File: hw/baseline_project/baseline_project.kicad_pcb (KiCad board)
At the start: 2 copper layers, 115 x 94 mm, 17 parts, among them J101 EXT_3V3, Q101 IRLD024PBF, SW101 UP, SW102 DOWN, SW103 LEFT, SW104 RIGHT, SW105 MODE, U101 EK-TM4C123GXL, U102 ESP8266-01/ESP-01, U103 Adafruit ST7735R

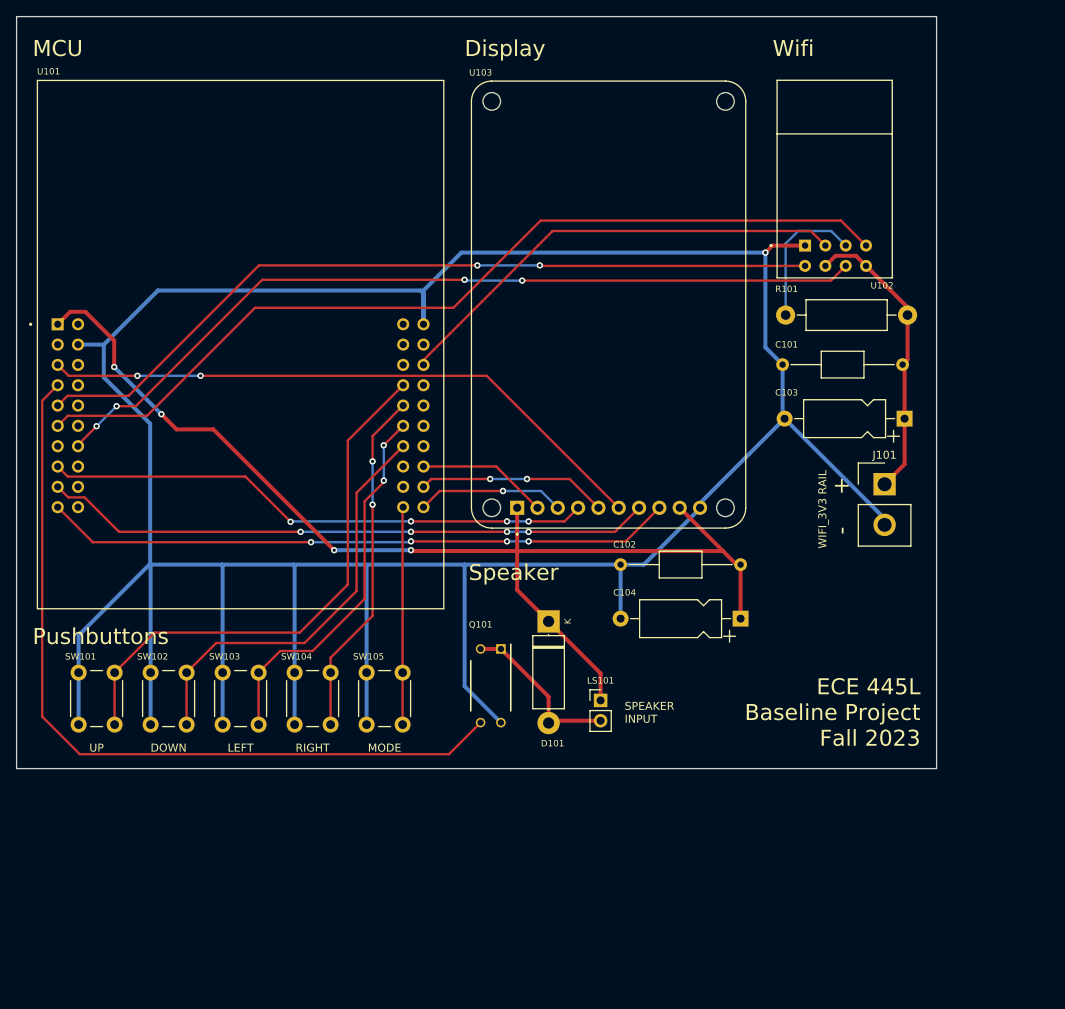
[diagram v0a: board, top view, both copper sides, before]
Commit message: SchematicDone
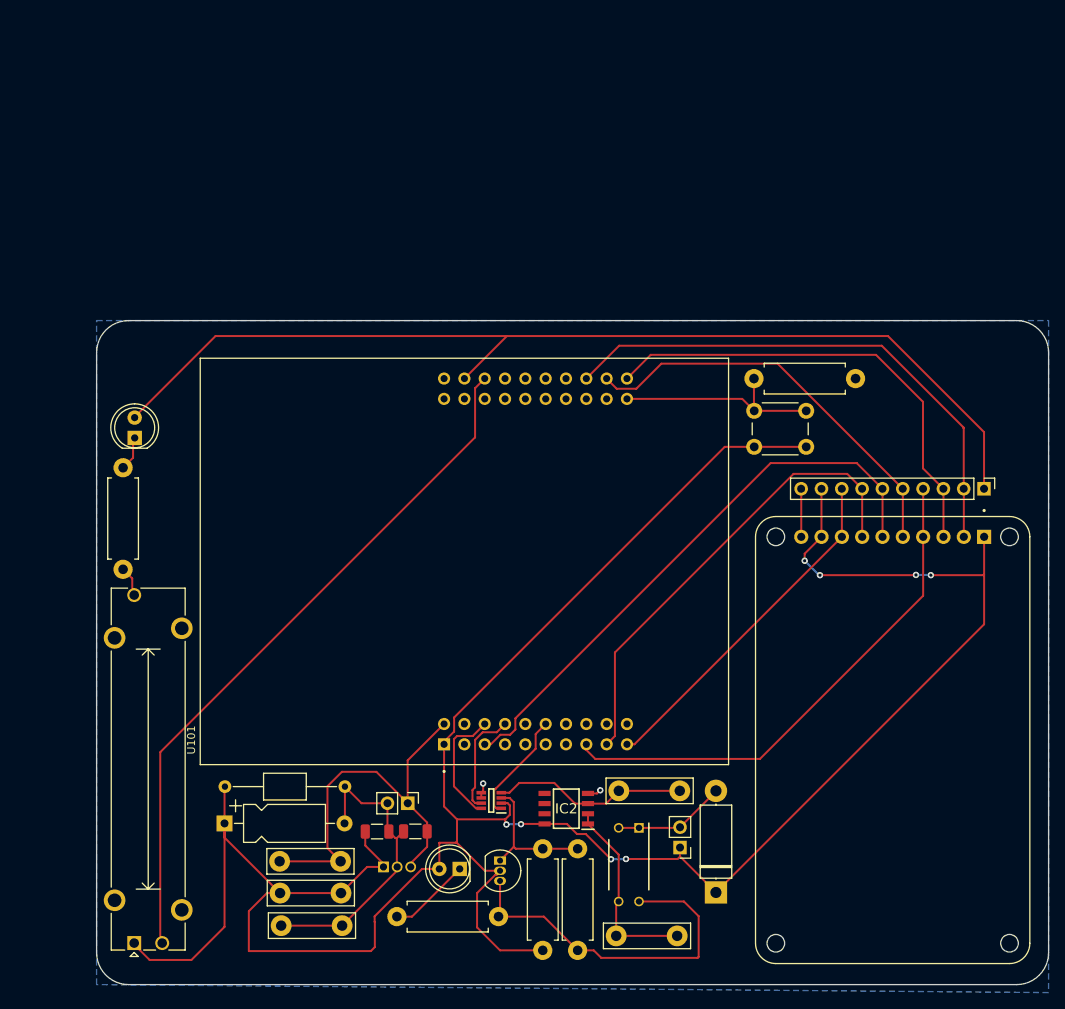
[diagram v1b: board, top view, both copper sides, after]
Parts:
- removed C101: 100nF, Capacitor_THT:C_Axial_L5.1mm_D3.1mm_P15.00mm_Horizontal
- removed C103: 4.7uF, Capacitor_THT:CP_Axial_L10.0mm_D4.5mm_P15.00mm_Horizontal
- removed J101: EXT_3V3, Connector_Samtec_HPM_THT:Samtec_HPM-02-01-x-S_Straight_1x02_Pitch5.08mm
- removed R101: 10k, Resistor_THT:R_Axial_DIN0411_L9.9mm_D3.6mm_P15.24mm_Horizontal
- removed SW101: UP, Button_Switch_THT:SW_PUSH_6mm
- removed SW102: DOWN, Button_Switch_THT:SW_PUSH_6mm
- removed SW103: LEFT, Button_Switch_THT:SW_PUSH_6mm
- removed SW104: RIGHT, Button_Switch_THT:SW_PUSH_6mm
- removed SW105: MODE, Button_Switch_THT:SW_PUSH_6mm
- removed U102: ESP8266-01/ESP-01, footprints:ai_thinker_ESP8266_01
- added C1: 1u, Capacitor_SMD:C_1206_3216Metric, F.Cu at (81.8, 132.8)
- added C2: 1u, Capacitor_SMD:C_1206_3216Metric, F.Cu at (77.1, 132.9)
- added D1: LED, LED_THT:LED_D5.0mm, F.Cu at (46.8, 83.7)
- added D2: LED, LED_THT:LED_D5.0mm, F.Cu at (87.4, 137.5)
- added IC1: AD5061BRJZ-1500RL7, footprints:SOT65P280X145-8N, F.Cu at (91.3, 129.0)
- added IC2: AD823ARZ, footprints:SOIC127P600X175-8N, F.Cu at (100.7, 130.0)
- added IC3: LP2950-33LPE3, footprints:TO127P419X482X788-3P, F.Cu at (78.3, 137.3)
- added J1: Logic, Connector_PinHeader_2.54mm:PinHeader_1x10_P2.54mm_Vertical, F.Cu at (152.9, 90.0)
- added J2: battery, Connector_PinHeader_2.54mm:PinHeader_1x02_P2.54mm_Vertical, F.Cu at (80.9, 129.3)
- added R1: R, Resistor_THT:R_Axial_DIN0411_L9.9mm_D3.6mm_P12.70mm_Horizontal, F.Cu at (45.3, 87.4)
- added R2: R, Resistor_THT:R_Axial_DIN0411_L9.9mm_D3.6mm_P12.70mm_Horizontal, F.Cu at (79.5, 143.5)
- added R3: R, Resistor_THT:R_Axial_DIN0411_L9.9mm_D3.6mm_P12.70mm_Horizontal, F.Cu at (97.8, 147.7)
- added R4: R, Resistor_THT:R_Axial_DIN0411_L9.9mm_D3.6mm_P12.70mm_Horizontal, F.Cu at (102.1, 135.0)
- added R5: R, Resistor_THT:R_Axial_DIN0411_L9.9mm_D3.6mm_P12.70mm_Horizontal, F.Cu at (124.2, 76.2)
- added RV1: R_Potentiometer, Potentiometer_THT:Potentiometer_Bourns_PTA3043_Single_Slide, F.Cu at (46.7, 146.8)
- added SW1: UP, Button_Switch_THT:SW_PUSH_6mm, F.Cu at (124.2, 80.3)
- added TP1: gnd, TestPoint:TestPoint_Bridge_Pitch7.62mm_Drill1.3mm, F.Cu at (65.1, 144.6)
- added TP2: 3v3, TestPoint:TestPoint_Bridge_Pitch7.62mm_Drill1.3mm, F.Cu at (64.9, 140.6)
- added TP3: vbat, TestPoint:TestPoint_Bridge_Pitch7.62mm_Drill1.3mm, F.Cu at (64.9, 136.6)
- added TP4: dacOut, TestPoint:TestPoint_Bridge_Pitch7.62mm_Drill1.3mm, F.Cu at (107.3, 127.8)
- added TP5: spkr, TestPoint:TestPoint_Bridge_Pitch7.62mm_Drill1.3mm, F.Cu at (107.0, 145.9)
- added U1: LM4041LP-ADJ, Package_TO_SOT_THT:TO-92_Inline, F.Cu at (92.4, 136.5)
- moved C102 70.2 mm to (58.0, 127.2), turned to 0 degrees
- moved C104 69.4 mm to (58.0, 131.8), turned to 0 degrees
- moved U103 65.0 mm to (141.5, 121.4), turned to -90 degrees
- moved D101 39.8 mm to (119.4, 140.5), turned to 90 degrees
- moved U101 39.0 mm to (88.0, 99.1), turned to 90 degrees
- moved Q101 28.2 mm to (108.5, 137.0)
- moved LS101 20.9 mm to (114.9, 134.9), turned to 180 degrees
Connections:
- U101 pad J1_4: /SPEAKER_GATE -> unconnected-(U101-PB1-PadJ1_4)
- U101 pad J1_5: /WIFI_TXD -> unconnected-(U101-PE4-PadJ1_5)
- U101 pad J1_6: /WIFI_RXD -> unconnected-(U101-PE5-PadJ1_6)
- U101 pad J2_2: unconnected-(U101-PB2-PadJ2_2) -> DebugOut
- U101 pad J2_3: /WIFI_IO2 -> AIN
- U101 pad J3_1: +5V -> +BATT
- U101 pad J3_3: unconnected-(U101-PD0-PadJ3_3) -> SS1_SCK
- U101 pad J3_4: unconnected-(U101-PD1-PadJ3_4) -> SS1_FS
- U101 pad J3_6: unconnected-(U101-PD3-PadJ3_6) -> SS1_MOSI
- U101 pad J3_7: /~{WIFI_RST} -> unconnected-(U101-PE1-PadJ3_7)
- U101 pad J4_4: /SW_UP -> unconnected-(U101-PC4-PadJ4_4)
- U101 pad J4_5: /SW_RIGHT -> unconnected-(U101-PC5-PadJ4_5)
- U101 pad J4_6: /SW_LEFT -> unconnected-(U101-PC6-PadJ4_6)
- U101 pad J4_7: /SW_DOWN -> unconnected-(U101-PC7-PadJ4_7)
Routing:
- net GND: track 392.9 -> 96.7 mm, vias 1 -> 2
- net +3V3: track 143.8 -> 341.3 mm, vias 4 -> 8
- net DebugOut: track 0.00 -> 130.2 mm
- net /WIFI_RXD: track 113.0 -> 0.00 mm
- net /~{WIFI_RST}: track 105.5 -> 0.00 mm, vias 4 -> 0
- net /WIFI_TXD: track 100.7 -> 0.00 mm, vias 2 -> 0
- net AIN: track 0.00 -> 87.3 mm
- net /SPEAKER_GATE: track 100.6 -> 24.6 mm
- net /SW_UP: track 68.0 -> 0.00 mm
- net /WIFI_IO2: track 58.3 -> 0.00 mm
- net /SW_DOWN: track 52.5 -> 0.00 mm
- net +BATT: track 0.00 -> 51.9 mm
- net /TFT_MISO: track 16.4 -> 66.8 mm
- net /SW_LEFT: track 47.2 -> 0.00 mm, vias 2 -> 0
- net /SW_RIGHT: track 43.6 -> 0.00 mm, vias 2 -> 0
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- added copper zone on B.Cu, net GND
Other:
- board size 115 x 94 mm -> 119 x 83 mm
- board text removed: "+"
- board text removed: "-"
- board text removed: "DOWN"
- board text removed: "Display"
- board text removed: "ECE 445L Baseline Project Fall 2023"
- board text removed: "LEFT"
- board text removed: "MCU"
- board text removed: "MODE"
- board text removed: "Pushbuttons"
- board text removed: "RIGHT"
- board text removed: "SPEAKER INPUT"
- board text removed: "Speaker"
- board text removed: "UP"
- board text removed: "WIFI_3V3 RAIL"
- board text removed: "Wifi"
